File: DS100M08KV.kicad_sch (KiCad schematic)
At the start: 128 parts, among them J1 wire2board, J10 BNC_panel_mount, J11 wire2board, J2 Conn_01x04_Socket, J3 wire2board, J4 wire2board, J8 red_safety_4mm_connector, J9 black_safety_4mm_connector, Q1 BD679, Q3 CMSN3416K-HF, Q4 BD680, Q5 CMSN3416K-HF, SW1 SW_DPDT_x2, SW2 SW_DPDT_x2, U1 AD8039, U2 AP9101CK6, U4 AD8009, U6 BQ21040DBV, U7 TLV61070ADBVR

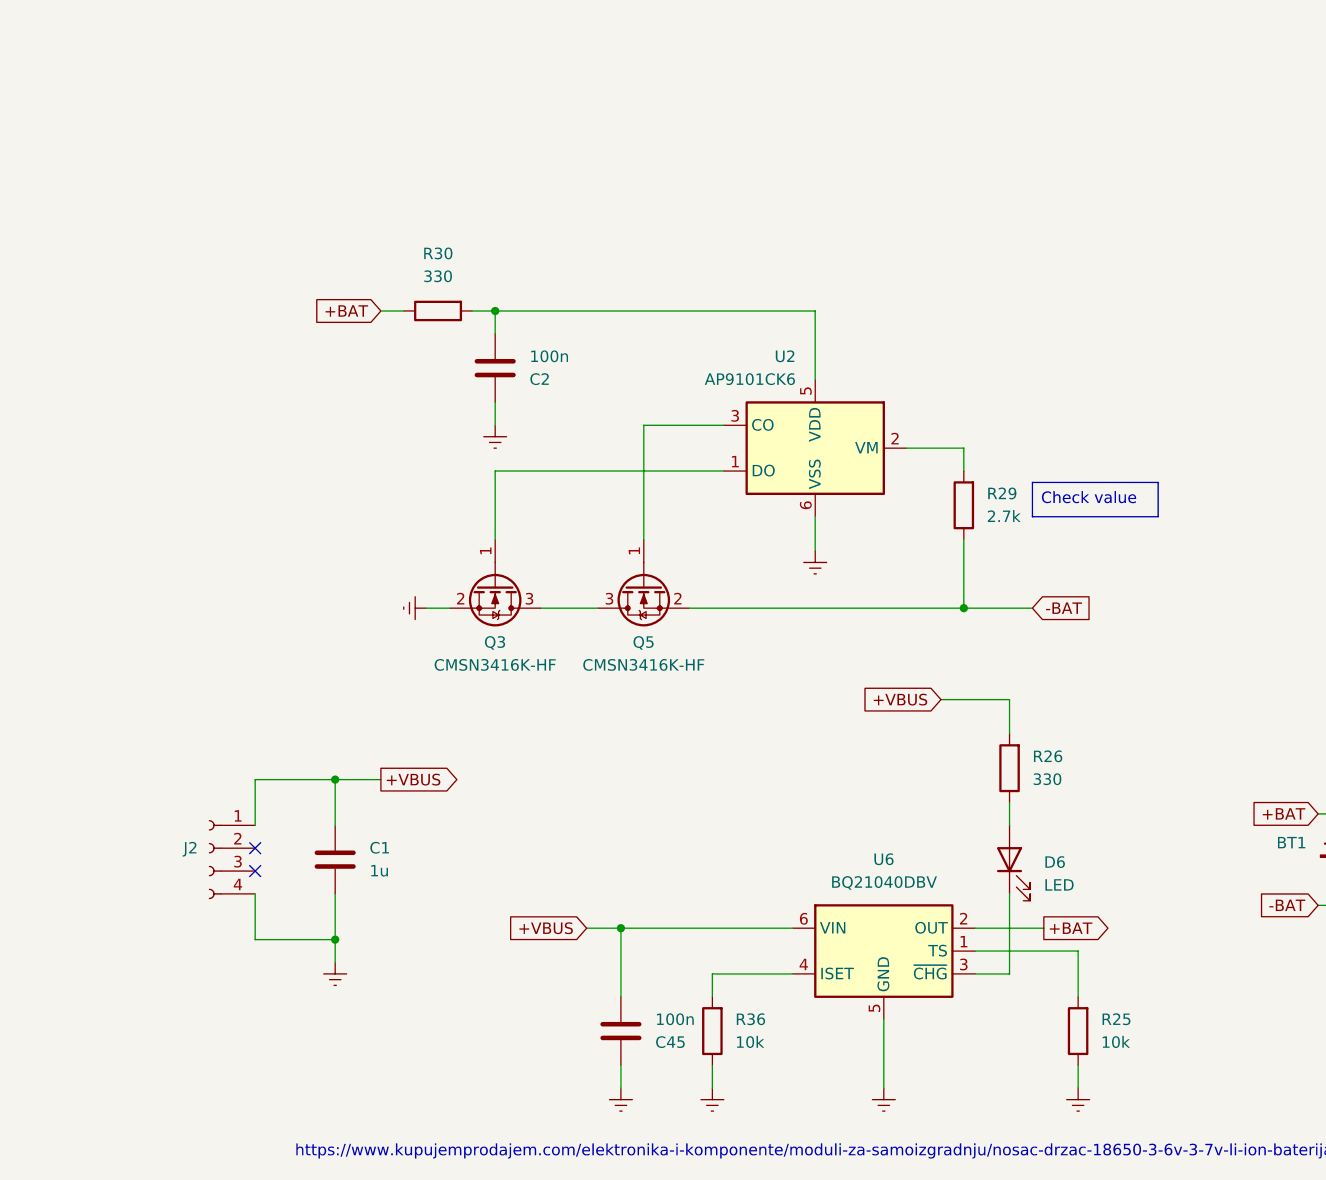
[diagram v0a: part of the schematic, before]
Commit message: Rutiranje gotovo.
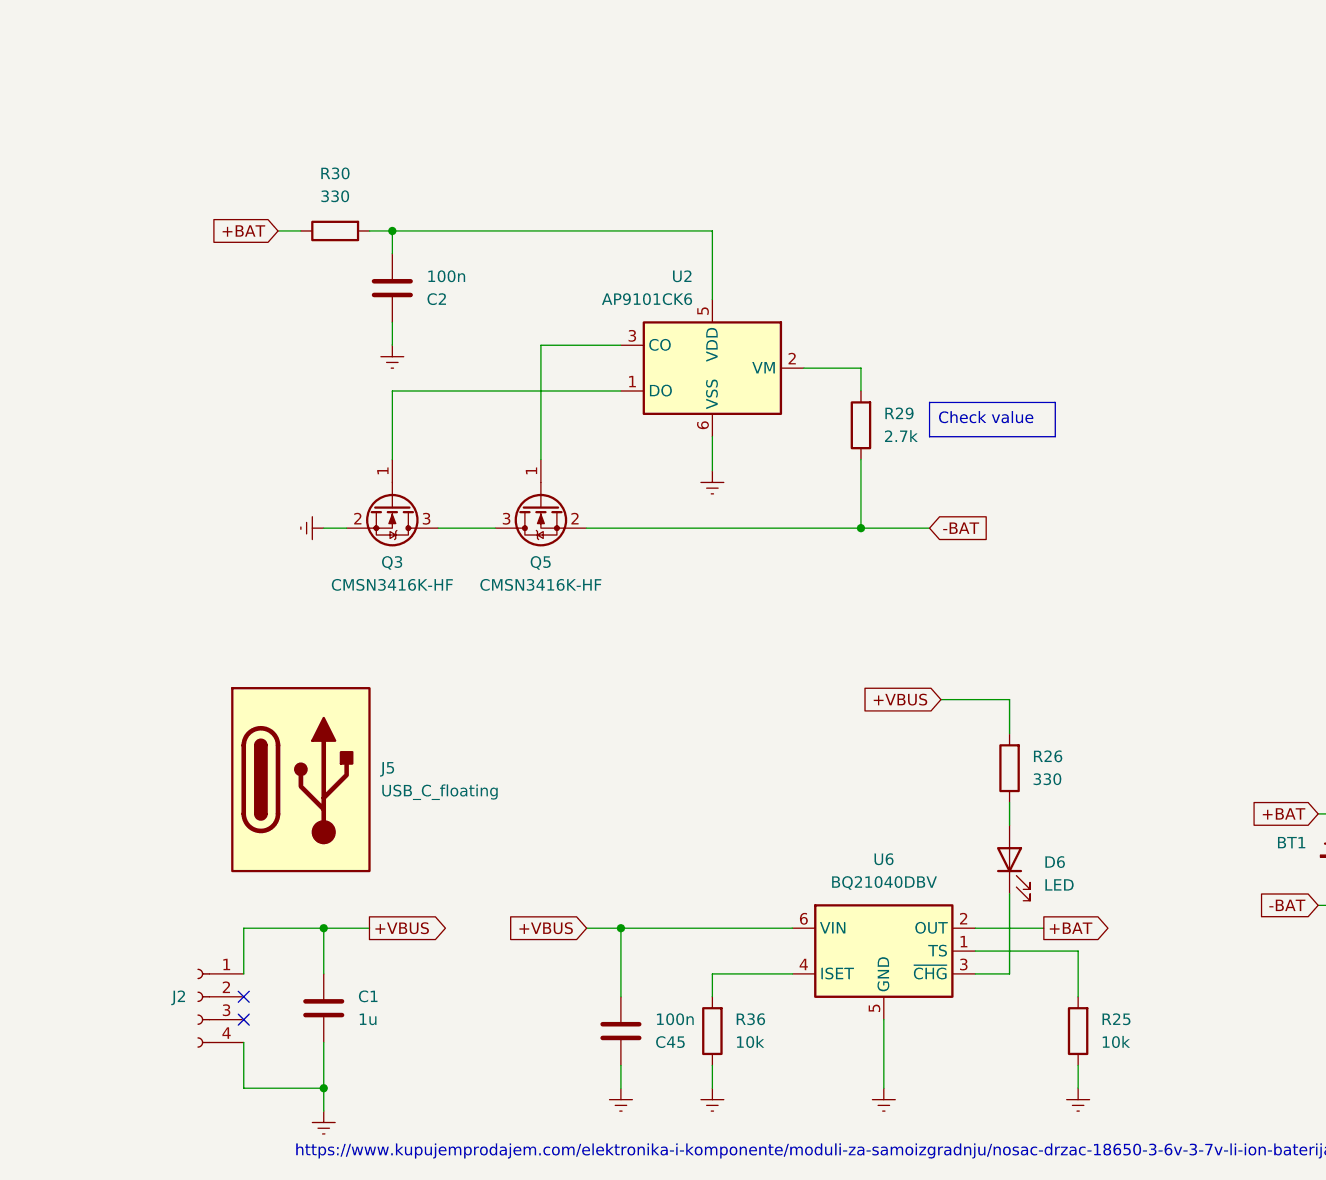
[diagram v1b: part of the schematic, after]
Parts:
- added J5: USB_C_floating, DS100M08KV:USB_C_floating, symbol DS100M08KV:USB_C_floating
- Q1, Q4: footprint DS100M08KV:TO-126-3_Horizontal_TabUp_No_Hole -> Package_TO_SOT_THT:TO-126-3_Vertical
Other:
- moved on the sheet: C1, C2, J2, Q3, Q5, R29, R30, U2
